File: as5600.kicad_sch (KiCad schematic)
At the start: 22 parts, among them J1 Conn_01x05_Socket, J2 Conn_01x12_Socket, J3 Conn_01x12_Socket, J4 Conn_01x05_Socket, J5 Conn_01x05_Socket, J6 Conn_01x05_Socket, J7 Conn_01x05_Socket, J8 Conn_01x05_Socket

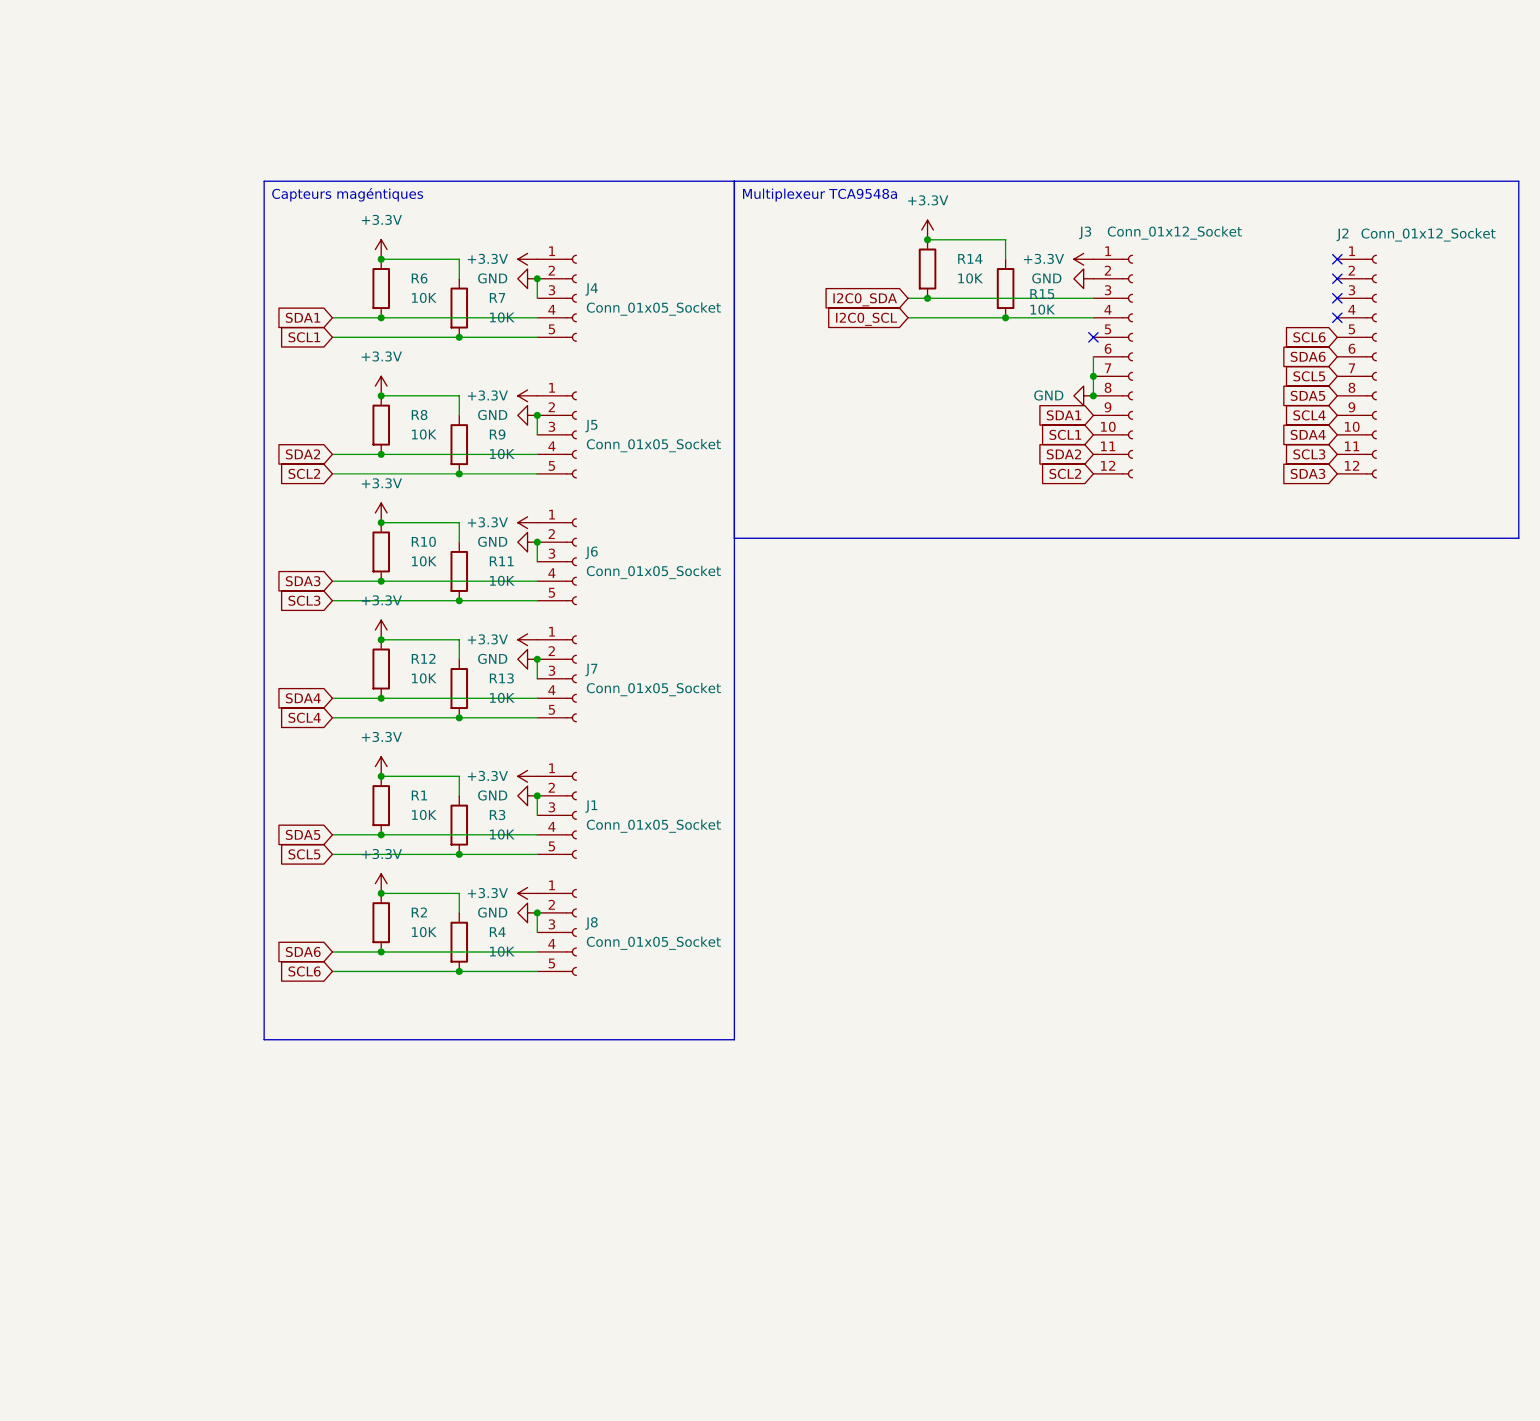
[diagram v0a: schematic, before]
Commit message: V1GD
V1 20/10/25
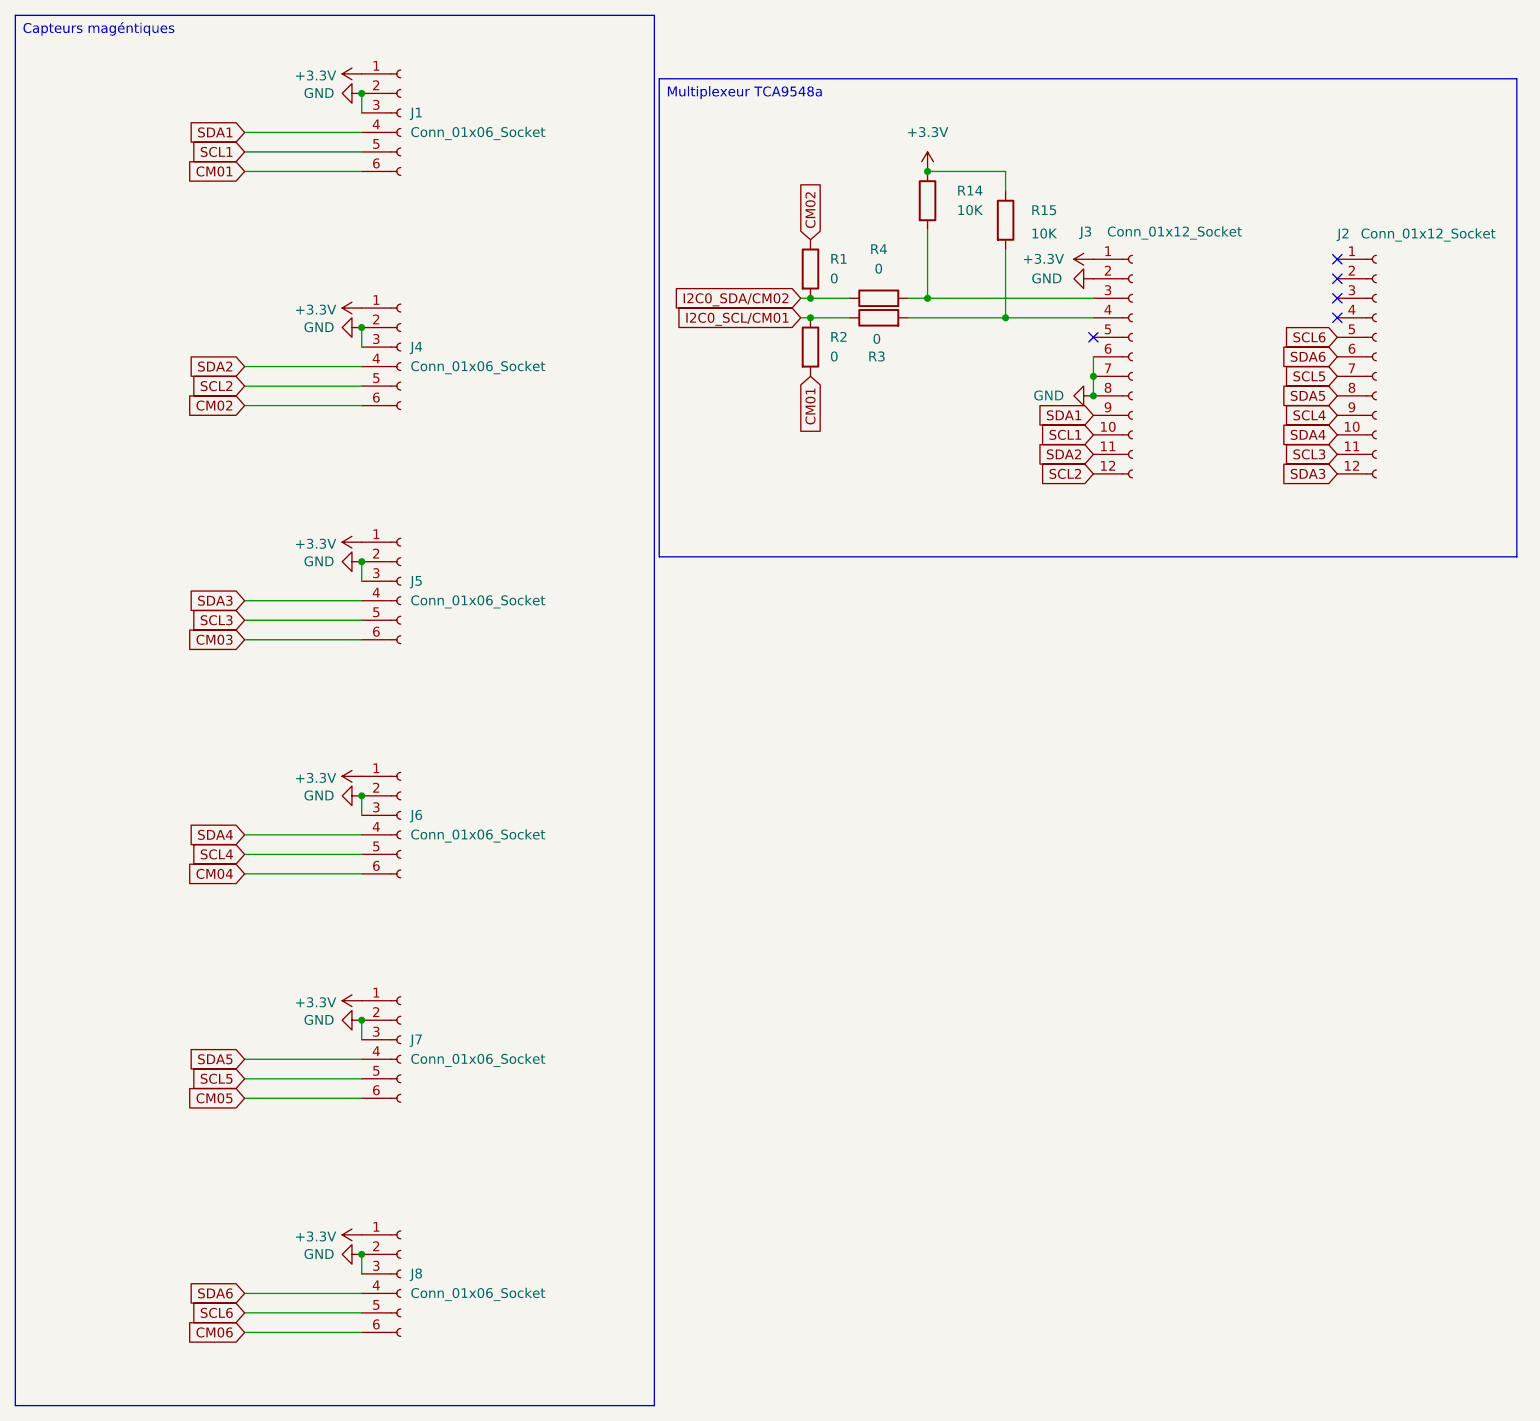
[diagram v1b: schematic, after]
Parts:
- removed J1, J4, J5, J6, J7, J8: Conn_01x05_Socket, Connector_JST:JST_EH_B5B-EH-A_1x05_P2.50mm_Vertical, symbol Connector:Conn_01x05_Socket
- removed R10, R11, R12, R13, R6, R7, R8, R9: 10K, Resistor_SMD:R_1206_3216Metric, symbol Device:R
- added J1, J4, J5, J6, J7, J8: Conn_01x06_Socket, Connector_PinHeader_2.54mm:PinHeader_1x06_P2.54mm_Vertical, symbol Connector:Conn_01x06_Socket
- R1, R2, R3, R4: value 10K -> 0
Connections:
- net +3.3V: now also J1.1 (Pin_1), J4.1 (Pin_1), J5.1 (Pin_1), J6.1 (Pin_1), J7.1 (Pin_1), J8.1 (Pin_1); no longer R1.1, R2.1, R3.1, R4.1
- net GND: now also J1.2 (Pin_2), J1.3 (Pin_3), J4.2 (Pin_2), J4.3 (Pin_3), J5.2 (Pin_2), J5.3 (Pin_3), J6.2 (Pin_2), J6.3 (Pin_3), J7.2 (Pin_2), J7.3 (Pin_3), J8.2 (Pin_2), J8.3 (Pin_3)
- net SCL1: now also J1.5 (Pin_5)
- net SCL2: now also J4.5 (Pin_5)
- net SCL3: now also J5.5 (Pin_5)
- net SCL4: now also J6.5 (Pin_5)
- net SCL5: now also J7.5 (Pin_5); no longer R3.2
- net SCL6: now also J8.5 (Pin_5); no longer R4.2
- net SDA1: now also J1.4 (Pin_4)
- net SDA2: now also J4.4 (Pin_4)
- net SDA3: now also J5.4 (Pin_4)
- net SDA4: now also J6.4 (Pin_4)
- net SDA5: now also J7.4 (Pin_4); no longer R1.2
- net SDA6: now also J8.4 (Pin_4); no longer R2.2
- net I2C0_SCL: no longer names the net of J3.4 (Pin_4), R15.2
- net I2C0_SCL: now also R3.2
- net I2C0_SDA: no longer names the net of J3.3 (Pin_3), R14.2
- net I2C0_SDA: now also R4.2
- new net CM01: J1.6 (Pin_6), R2.2
- new net CM02: J4.6 (Pin_6), R1.1
- new net CM03: J5.6 (Pin_6)
- new net CM04: J6.6 (Pin_6)
- new net CM05: J7.6 (Pin_6)
- new net CM06: J8.6 (Pin_6)
- new net I2C0_SCL/CM01: R2.1, R3.1
- new net I2C0_SDA/CM02: R1.2, R4.1
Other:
- moved on the sheet: R14, R15
